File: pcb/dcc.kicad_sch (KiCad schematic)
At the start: 23 parts

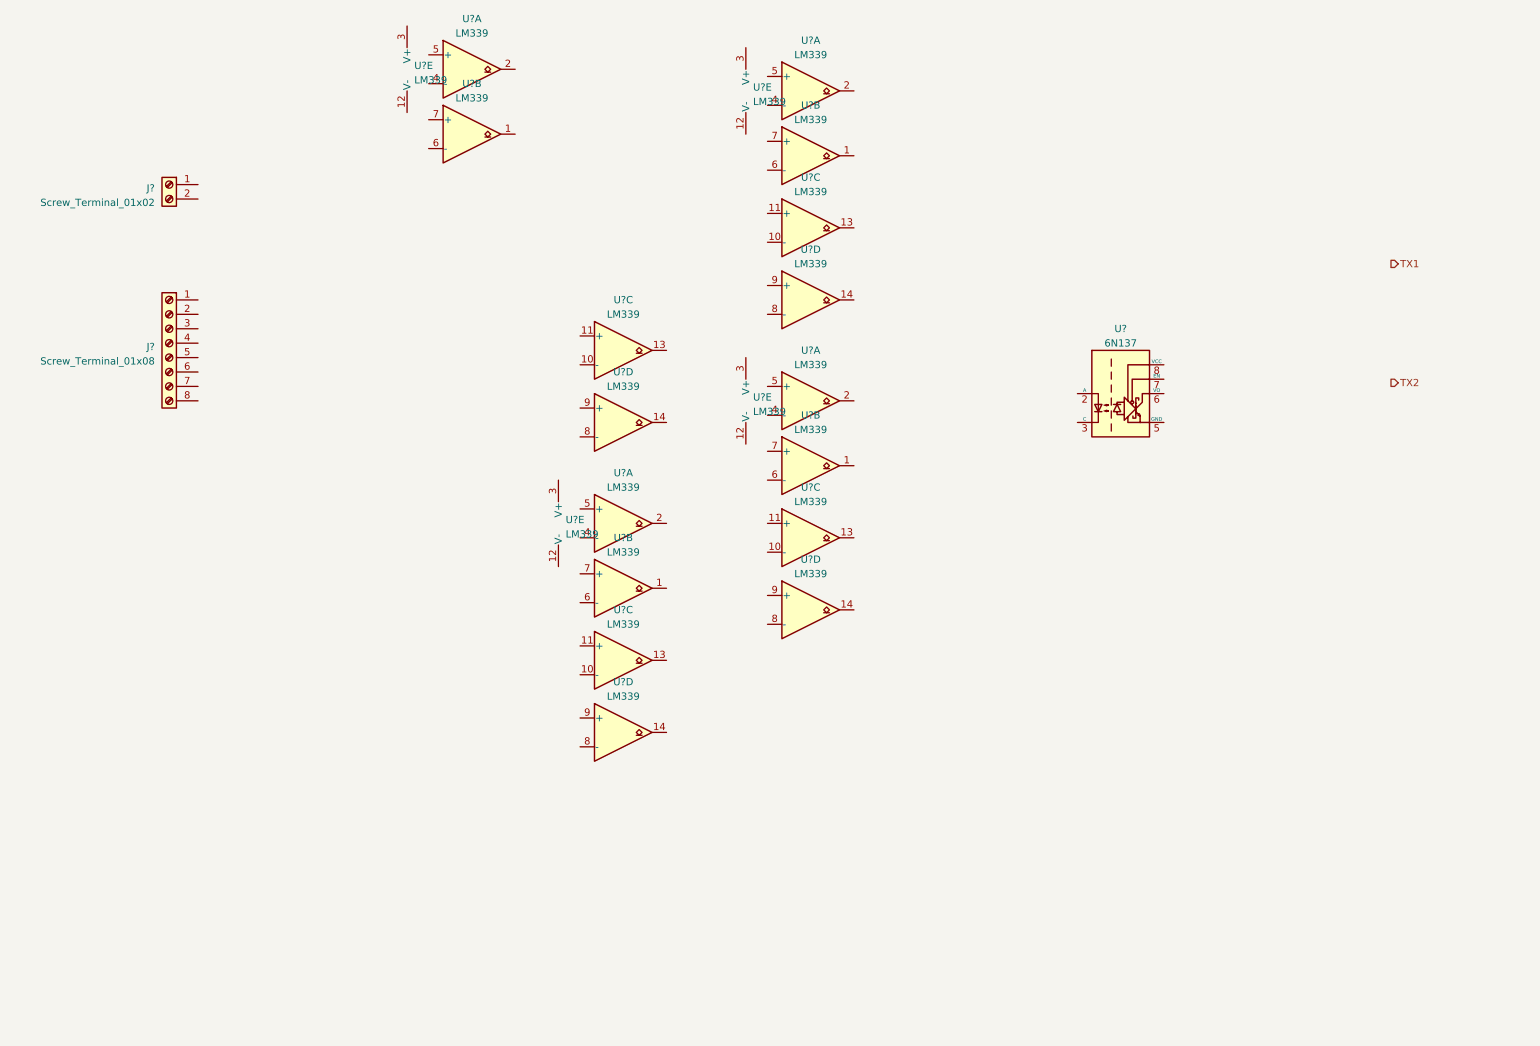
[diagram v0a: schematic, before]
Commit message: Finished MTB part.
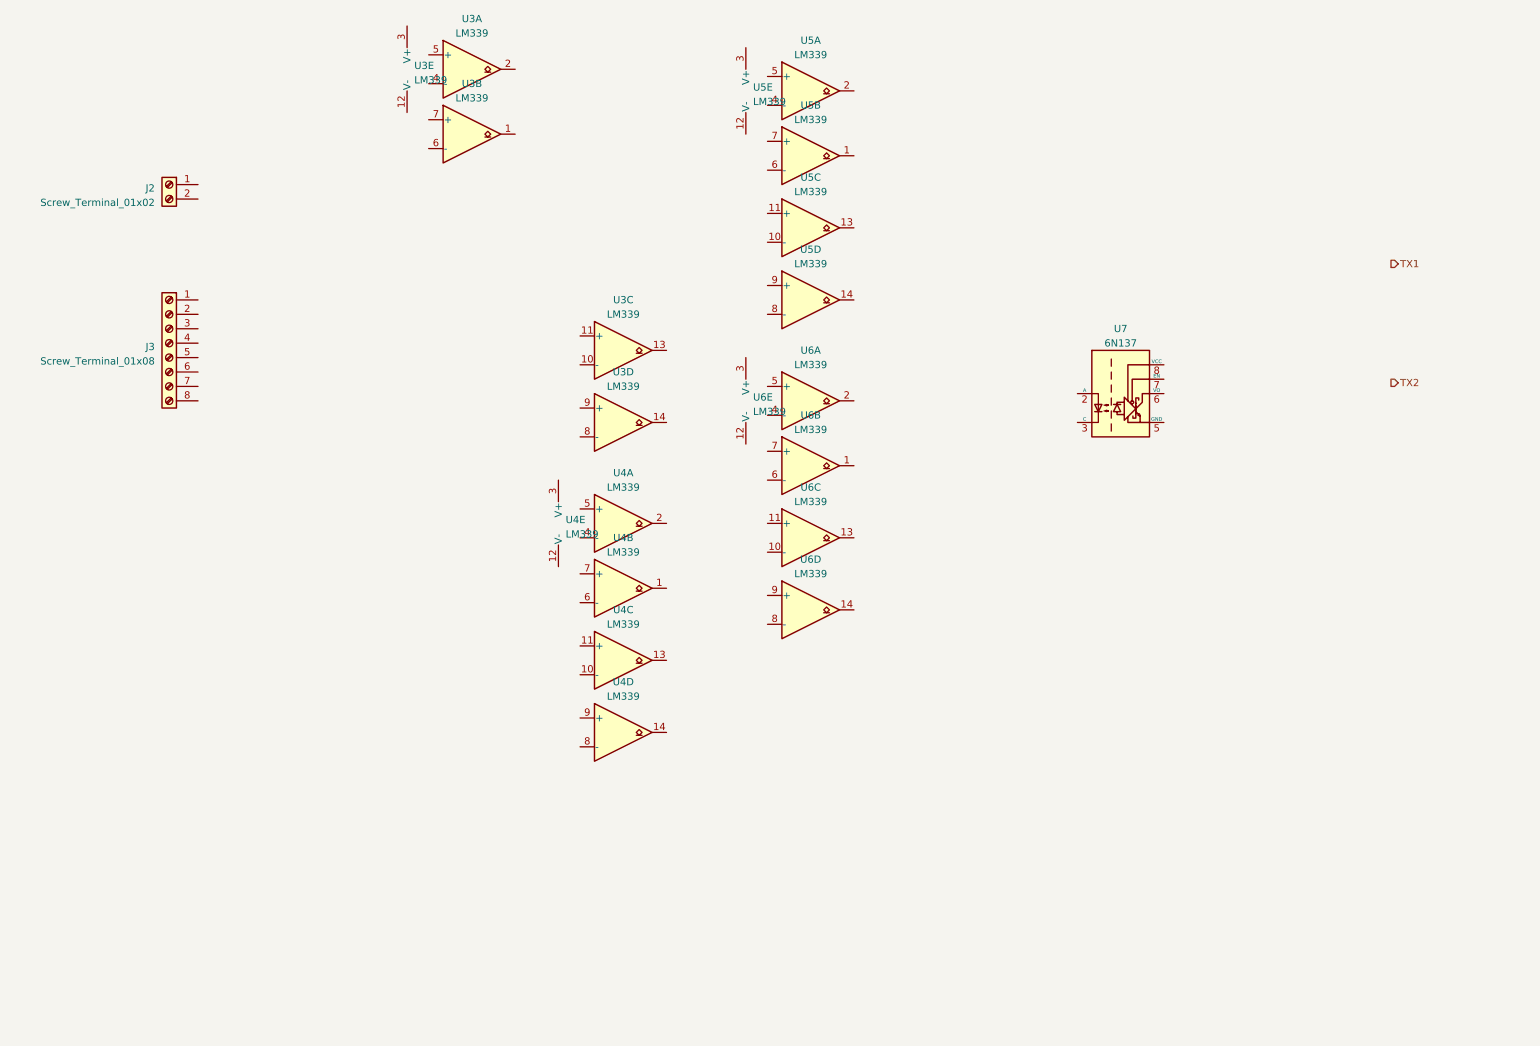
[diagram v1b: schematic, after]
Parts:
- gave numbers to parts that had none: 7

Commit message: DCC WIP.
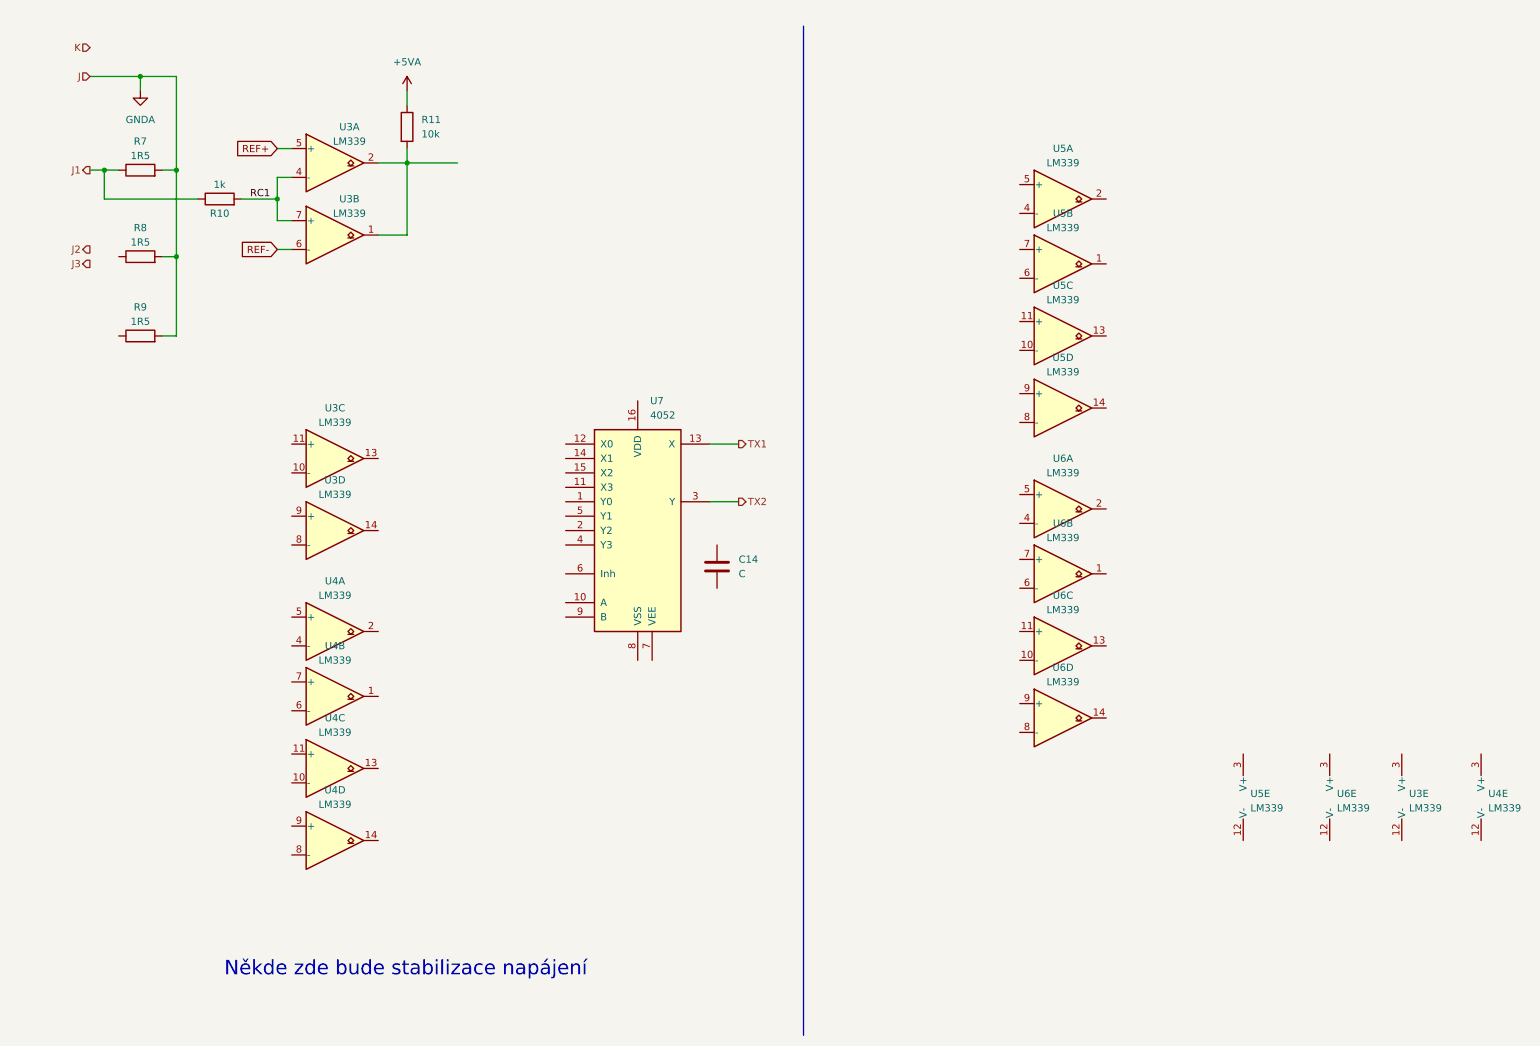
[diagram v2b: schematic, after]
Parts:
- removed J2: Screw_Terminal_01x02, symbol Connector:Screw_Terminal_01x02
- removed J3: Screw_Terminal_01x08, symbol Connector:Screw_Terminal_01x08
- removed U7: 6N137, Package_DIP:DIP-8_W7.62mm, symbol Isolator:6N137
- added C14: C, symbol Device:C
- added R10: 1k, symbol Device:R
- added R11: 10k, symbol Device:R
- added R7, R8, R9: 1R5, symbol Device:R
- added U7: 4052, symbol 4xxx:4052
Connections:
- net TX1: now also U7.13 (X)
- net TX2: now also U7.3 (Y)
- net at U3.2: now also U3.1, R11.2
- net RC1: now reaches U3.4 (-)
- net RC1: now also U3.7 (+), R10.2
- net REF+: now reaches U3.5 (+)
- net REF-: now reaches U3.6 (-)
- new net +5VA: R11.1
- new net GNDA: R7.2, R8.2, R9.2
- new net J1: R10.1, R7.1
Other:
- note added: "Někde zde bude stabilizace napájení"
- moved on the sheet: U3A, U3B, U3C, U3D, U3E, U4A, U4B, U4C, U4D, U4E, U5A, U5B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
